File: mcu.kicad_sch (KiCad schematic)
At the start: 1 part, among them U1 RP2040

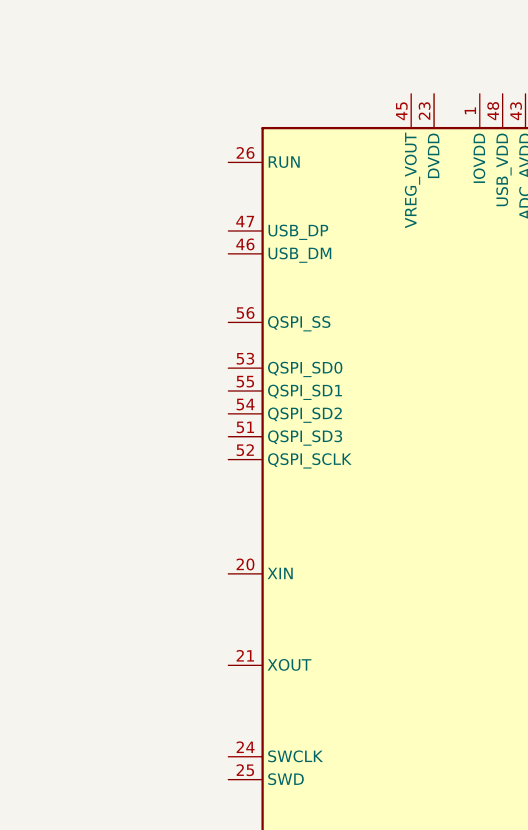
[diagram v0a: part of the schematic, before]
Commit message: adding labels and updating PCB
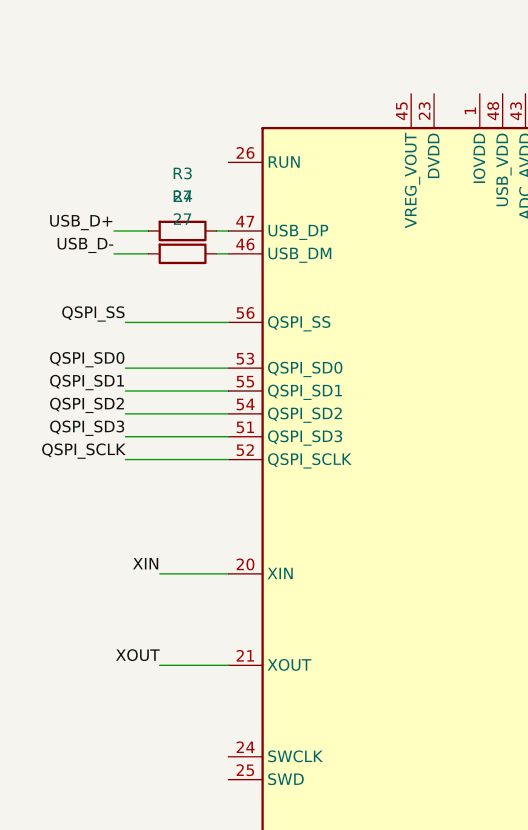
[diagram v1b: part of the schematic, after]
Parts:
- added R3, R4: 27, Resistor_SMD:R_0508_1220Metric, symbol Device:R
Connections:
- net XIN: now reaches U1.20 (XIN)
- net XOUT: now reaches U1.21 (XOUT)
- net at U1.46 (USB_DM): now also R4.1
- net at U1.47 (USB_DP): now also R3.1
- net QSPI_SD3: now reaches U1.51 (QSPI_SD3)
- net QSPI_SCLK: now reaches U1.52 (QSPI_SCLK)
- net QSPI_SD0: now reaches U1.53 (QSPI_SD0)
- net QSPI_SD2: now reaches U1.54 (QSPI_SD2)
- net QSPI_SD1: now reaches U1.55 (QSPI_SD1)
- net QSPI_SS: now reaches U1.56 (QSPI_SS)
- new net USB_D+: R3.2
- new net USB_D-: R4.2
